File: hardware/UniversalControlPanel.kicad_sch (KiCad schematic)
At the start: 63 parts, among them IC1 PSM712-LF-T7, J1 Conn_01x09, J10 Conn_01x02, J2 Conn_01x09, J3 Conn_01x40, J4 Conn_02x03_Odd_Even, J5 Conn_01x03, J6 Conn_01x07, J9 Conn_01x02, Q1 2N7002, Q2 2N7002, Q3 2N7002, SW1 SW_Push, U1 TSR_1-2433, U2 MAX14783ExS, U3 L78L05_SOT89, U5 SN65HVD230, U6 ESP32-S2-WROOM-I

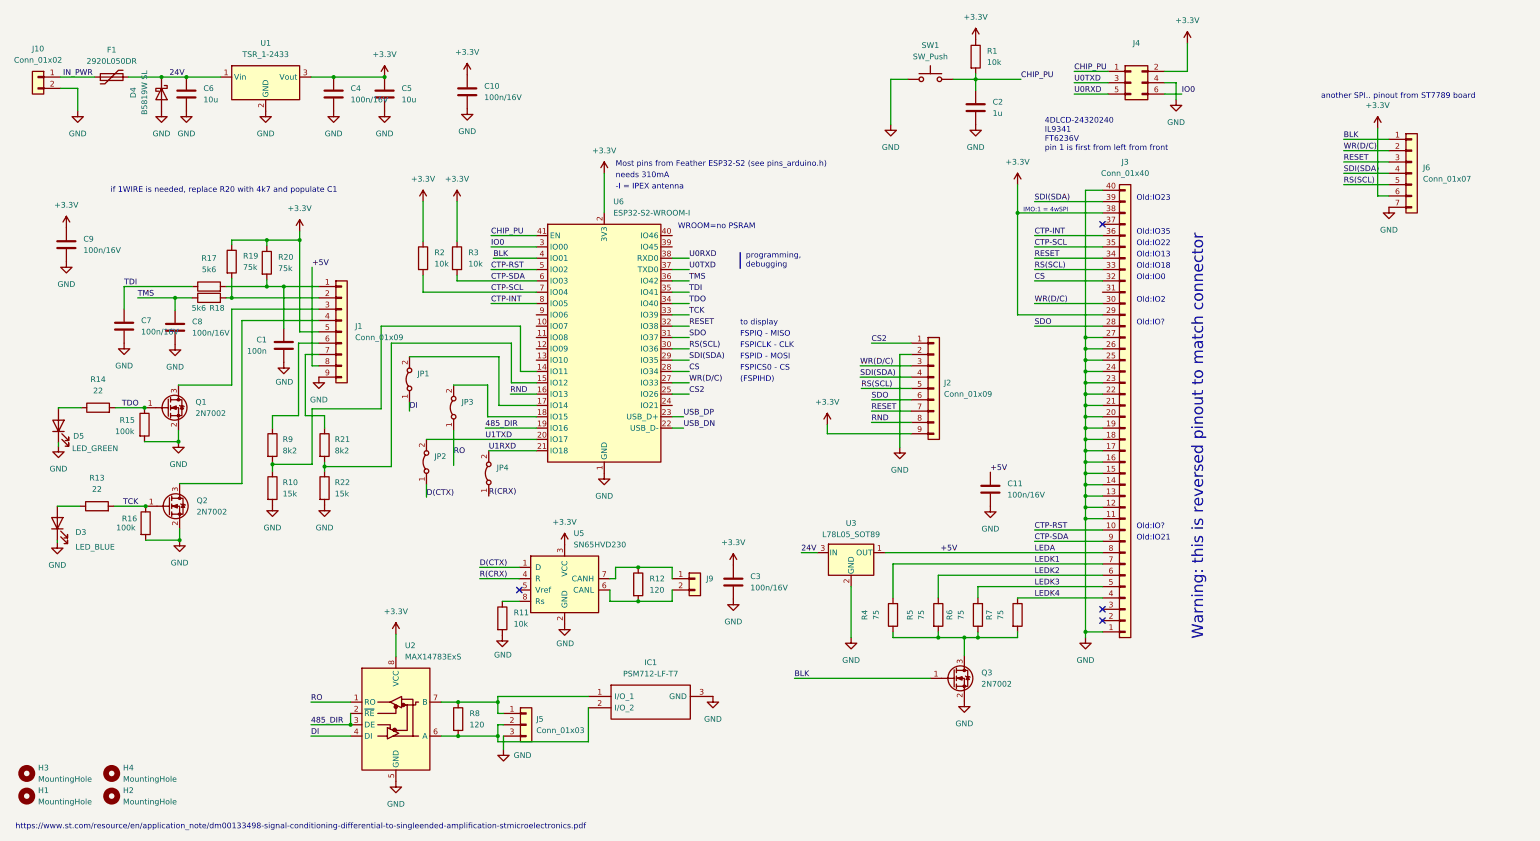
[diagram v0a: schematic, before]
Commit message: report
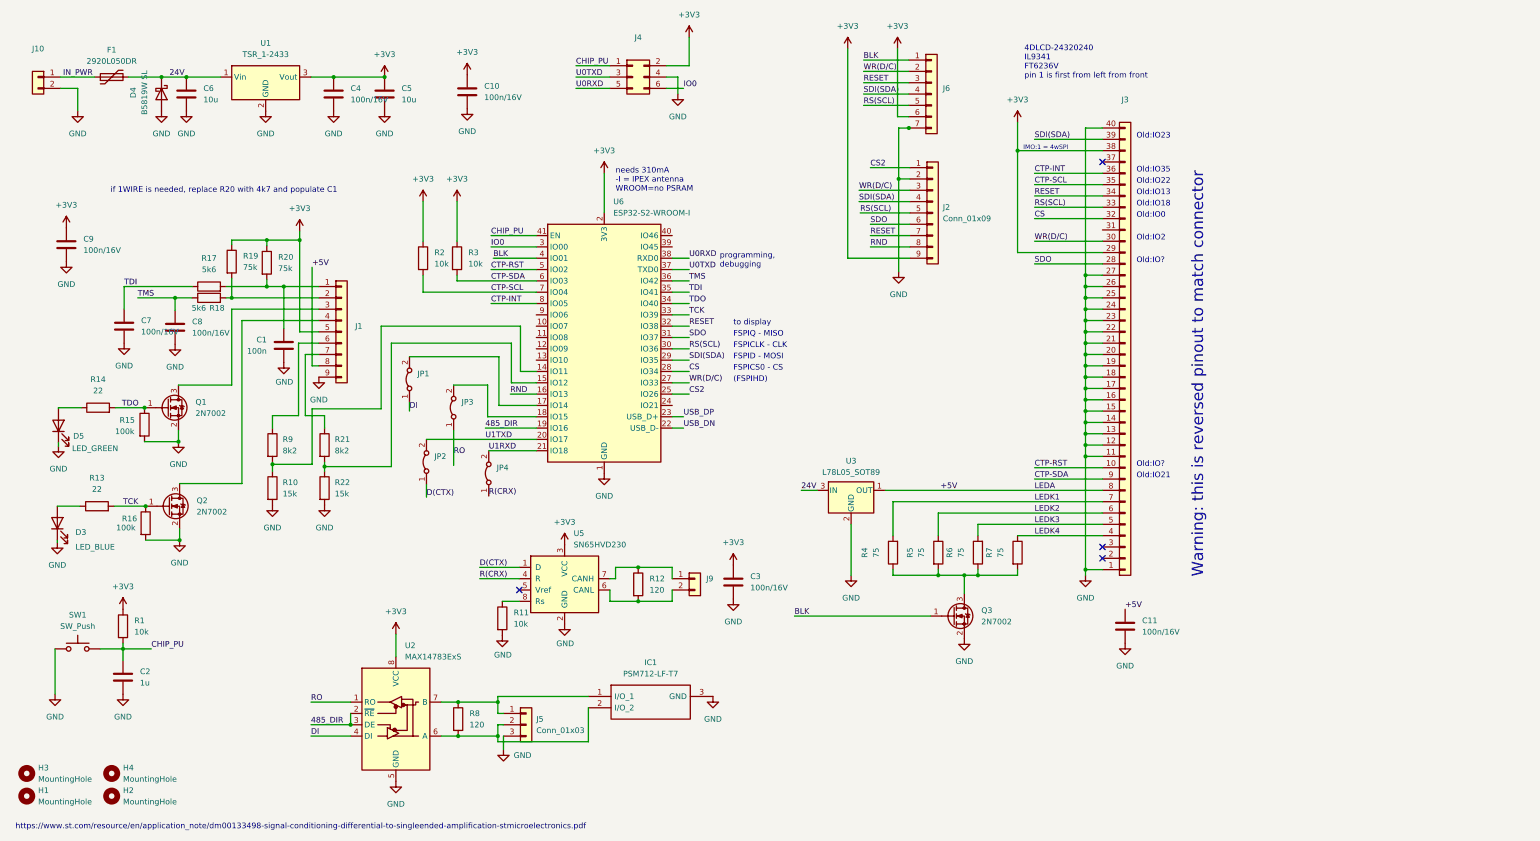
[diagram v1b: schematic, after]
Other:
- note added: "needs 310mA -I = IPEX antenna WROOM=no PSRAM"
- note removed: "-I = IPEX antenna"
- note removed: "Most pins from Feather ESP32-S2 (see pins_arduino.h)"
- note removed: "WROOM=no PSRAM"
- note removed: "another SPI.. pinout from ST7789 board"
- note removed: "needs 310mA"
- moved on the sheet: C11, C2, J2, J3, J4, J6, Q3, R1, R4, R5, R6, R7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
